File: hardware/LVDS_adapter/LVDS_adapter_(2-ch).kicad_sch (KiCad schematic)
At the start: 10 parts, among them J1 DF12NB(3.0)-30DS-0.5V(51), J2 LVDS, J3 BAKLIGHT_POWER

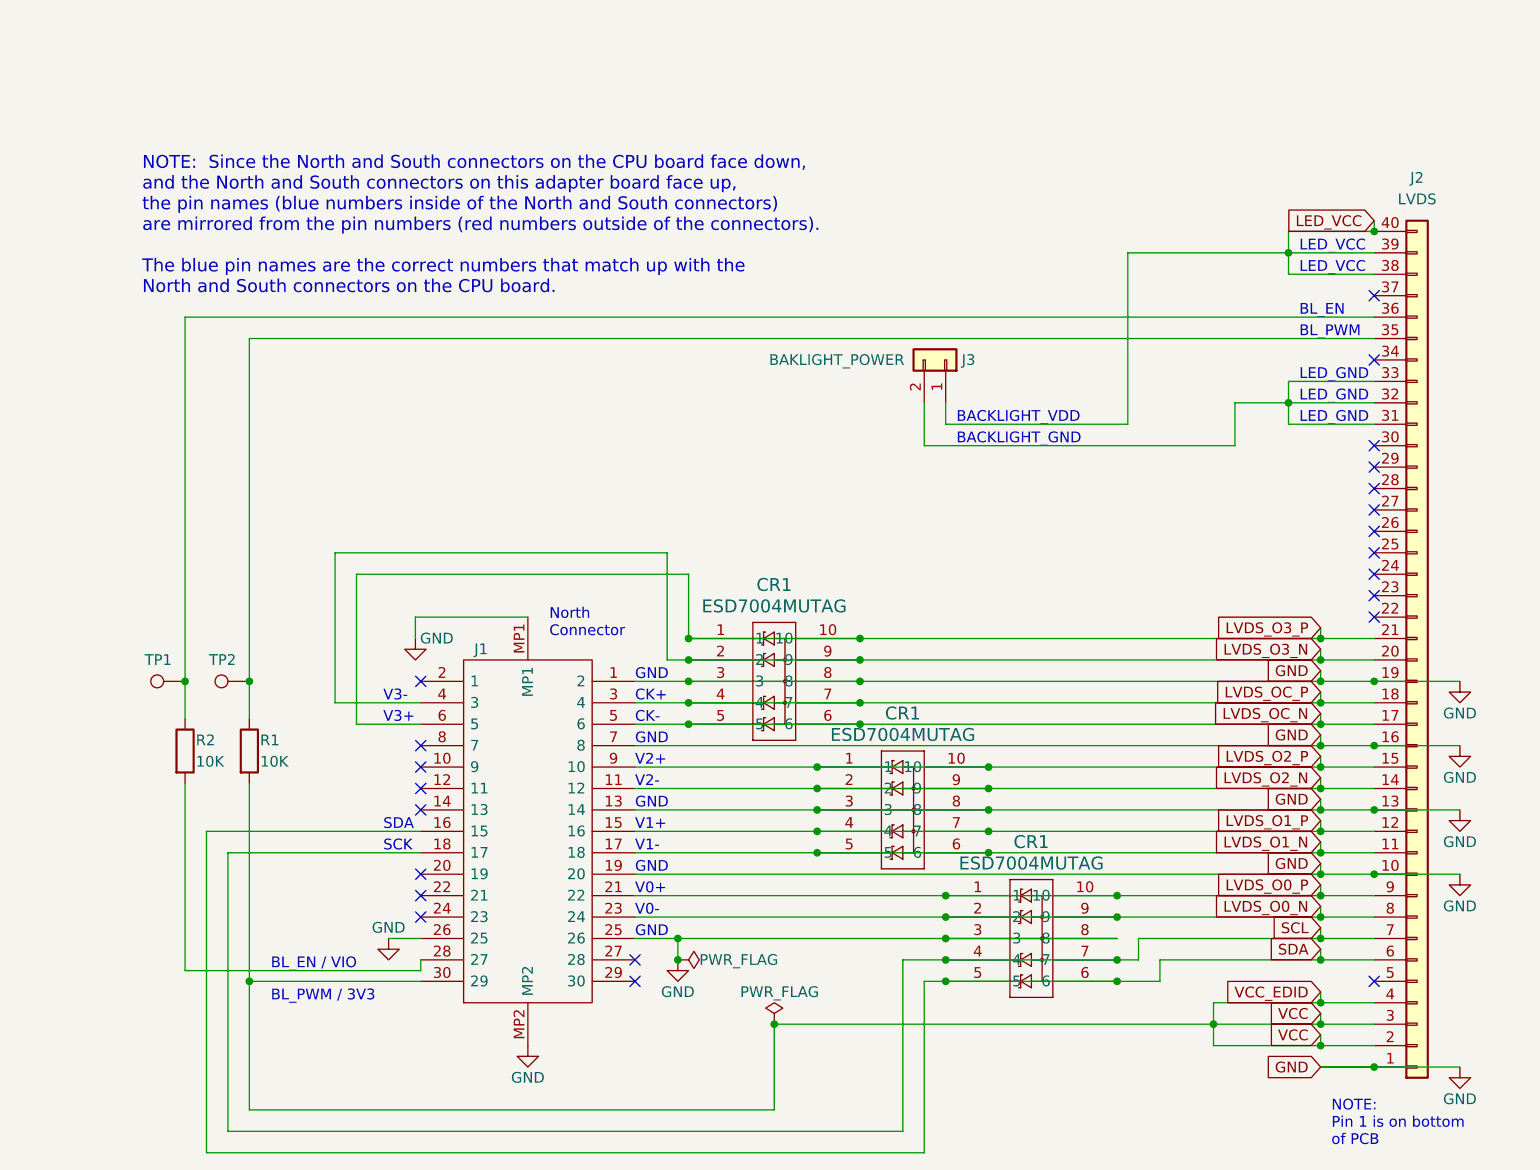
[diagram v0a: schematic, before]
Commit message: update PCB design files
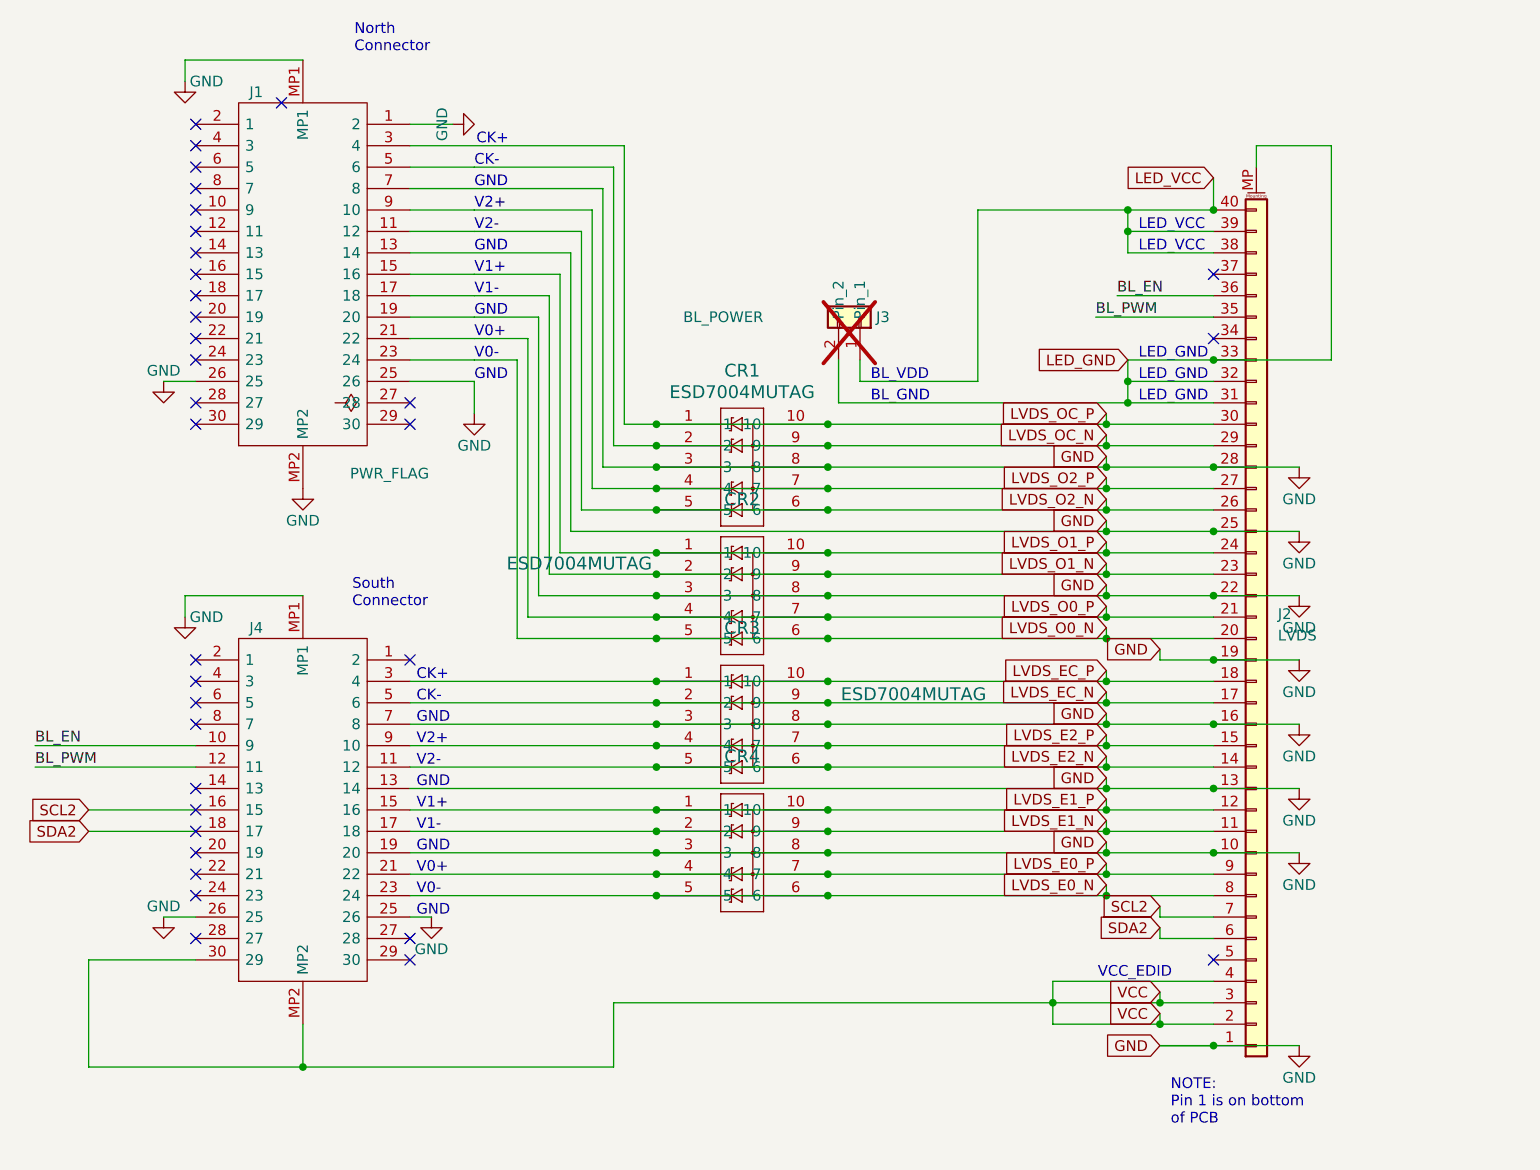
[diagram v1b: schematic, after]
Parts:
- removed CR1 (x3): ESD7004MUTAG, ESD7004:UDFN10_517BB_ONS-L, symbol ESD7004:ESD7004MUTAG
- removed R1, R2: 10K, Resistor_SMD:R_0402_1005Metric, symbol Device:R
- removed TP1, TP2: TestPoint, TestPoint:TestPoint_Pad_1.0x1.0mm, symbol Connector:TestPoint
- added CR1, CR2, CR3, CR4: ESD7004MUTAG, ESD7004:UDFN10_517BB_ONS-L, symbol ESD7004:ESD7004MUTAG
- added J4: DF12NB(3.0)-30DS-0.5V(51), Library:DF12NB3030DP05V51, symbol DF12NB_3.0_-30DP-0.5V_51_:DF12NB_3.0_-30DP-0.5V_51_
- J2: footprint Connector_FFC-FPC:Hirose_FH12-40S-0.5SH_1x40-1MP_P0.50mm_Horizontal -> Library:FPC-SMD_40P-P0.50_L4.4-W25.6; symbol Connector_Generic:Conn_01x40 -> Connector_Generic_MountingPin:Conn_01x40_MountingPin
- J3: value BAKLIGHT_POWER -> BL_POWER; now not fitted
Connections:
- net GND: now also J2.22 (Pin_22), J2.25 (Pin_25), J2.28 (Pin_28), CR1.3, CR1.8, CR2.3, CR2.8, CR3.3, CR3.8, CR4.3, CR4.8, J4.13 (14), J4.19 (20), J4.25 (26), J4.26 (25), J4.7 (8), J4.MP1
- net LVDS_O0_N: now also J2.20 (Pin_20), CR2.5, CR2.6; no longer J2.8 (Pin_8)
- net LVDS_O0_P: now also J2.21 (Pin_21), CR2.4, CR2.7; no longer J2.9 (Pin_9)
- net LVDS_O1_N: now also J2.23 (Pin_23), CR2.2, CR2.9; no longer J2.11 (Pin_11)
- net LVDS_O1_P: now also J2.24 (Pin_24), CR2.1, CR2.10; no longer J2.12 (Pin_12)
- net LVDS_O2_N: now also J2.26 (Pin_26), CR1.5, CR1.6; no longer J2.14 (Pin_14)
- net LVDS_O2_P: now also J2.27 (Pin_27), CR1.4, CR1.7; no longer J2.15 (Pin_15)
- net LVDS_OC_N: now also J2.29 (Pin_29), CR1.2, CR1.9; no longer J2.17 (Pin_17)
- net LVDS_OC_P: now also J2.30 (Pin_30), CR1.1, CR1.10; no longer J2.18 (Pin_18)
- net VCC: now also J4.30 (29), J4.MP2; no longer J1.30 (29)
- net LED_GND: now reaches J2.31 (Pin_31), J2.32 (Pin_32), J2.33 (Pin_33), J3.2 (Pin_2)
- net LED_GND: now also J2.MP (MountPin)
- net BL_PWM: now reaches J2.35 (Pin_35)
- net BL_PWM: now also J4.12 (11)
- net BL_EN: now reaches J2.36 (Pin_36)
- net BL_EN: now also J4.10 (9)
- net LVDS_O3_N: no longer names the net of J1.4 (3)
- net LVDS_O3_N: no longer J2.20 (Pin_20)
- net LVDS_O3_P: no longer names the net of J1.6 (5)
- net LVDS_O3_P: no longer J2.21 (Pin_21)
- net SCL: no longer names the net of J1.18 (17)
- net SCL: no longer J2.7 (Pin_7)
- net SDA: no longer names the net of J1.16 (15)
- net SDA: no longer J2.6 (Pin_6)
- new net LVDS_E0_N: CR4.5, CR4.6, J2.8 (Pin_8), J4.23 (24)
- new net LVDS_E0_P: CR4.4, CR4.7, J2.9 (Pin_9), J4.21 (22)
- new net LVDS_E1_N: CR4.2, CR4.9, J2.11 (Pin_11), J4.17 (18)
- new net LVDS_E1_P: CR4.1, CR4.10, J2.12 (Pin_12), J4.15 (16)
- new net LVDS_E2_N: CR3.5, CR3.6, J2.14 (Pin_14), J4.11 (12)
- new net LVDS_E2_P: CR3.4, CR3.7, J2.15 (Pin_15), J4.9 (10)
- new net LVDS_EC_N: CR3.2, CR3.9, J2.17 (Pin_17), J4.5 (6)
- new net LVDS_EC_P: CR3.1, CR3.10, J2.18 (Pin_18), J4.3 (4)
- new net SCL2: J2.7 (Pin_7), J4.16 (15)
- new net SDA2: J2.6 (Pin_6), J4.18 (17)
- no-connect marks 22 -> 34
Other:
- note added: "BL_GND"
- note added: "BL_VDD"
- note added: "South Connector"
- note added: "VCC_EDID"
- note removed: "BACKLIGHT_GND"
- note removed: "BACKLIGHT_VDD"
- note removed: "BL_EN"
- note removed: "BL_EN / VIO"
- note removed: "BL_PWM"
- note removed: "BL_PWM / 3V3"
- note removed: "NOTE: Since the North and South connectors on the CPU board face down, and the North and South connectors on this adapter board face up, the pin names (blue numbers inside of the North and South connectors) are mirrored from the pin numbers (red numbers outside of the connectors). The blue pin names are the correct numbers that match up with the North and South connectors on the CPU board."
- note removed: "SCK"
- note removed: "SDA"
- note removed: "V3+"
- note removed: "V3-"
- title: LVDS adapter board -> LVDS adapter board - 2ch
